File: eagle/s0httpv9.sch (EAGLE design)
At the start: 32 parts, among them X1 MKDSN1,5/6-5,08, X2 MKDSN1,5/6-5,08

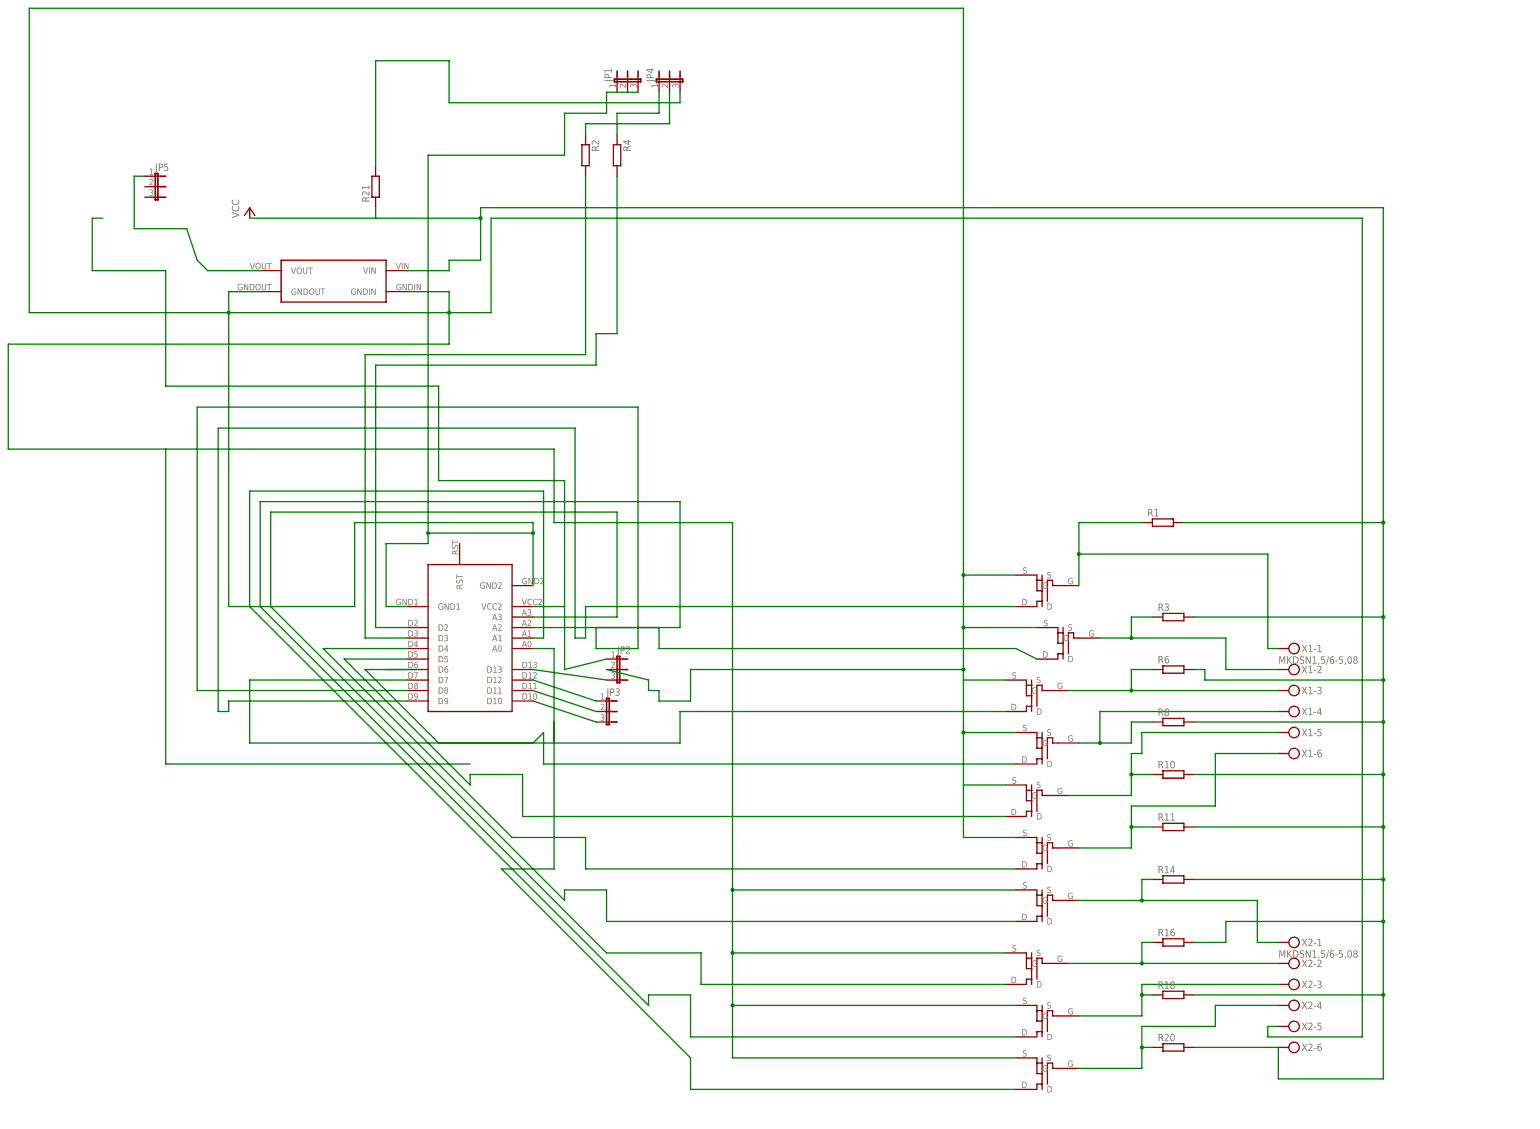
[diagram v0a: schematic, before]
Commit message: schematic cleanup and tagging as v9
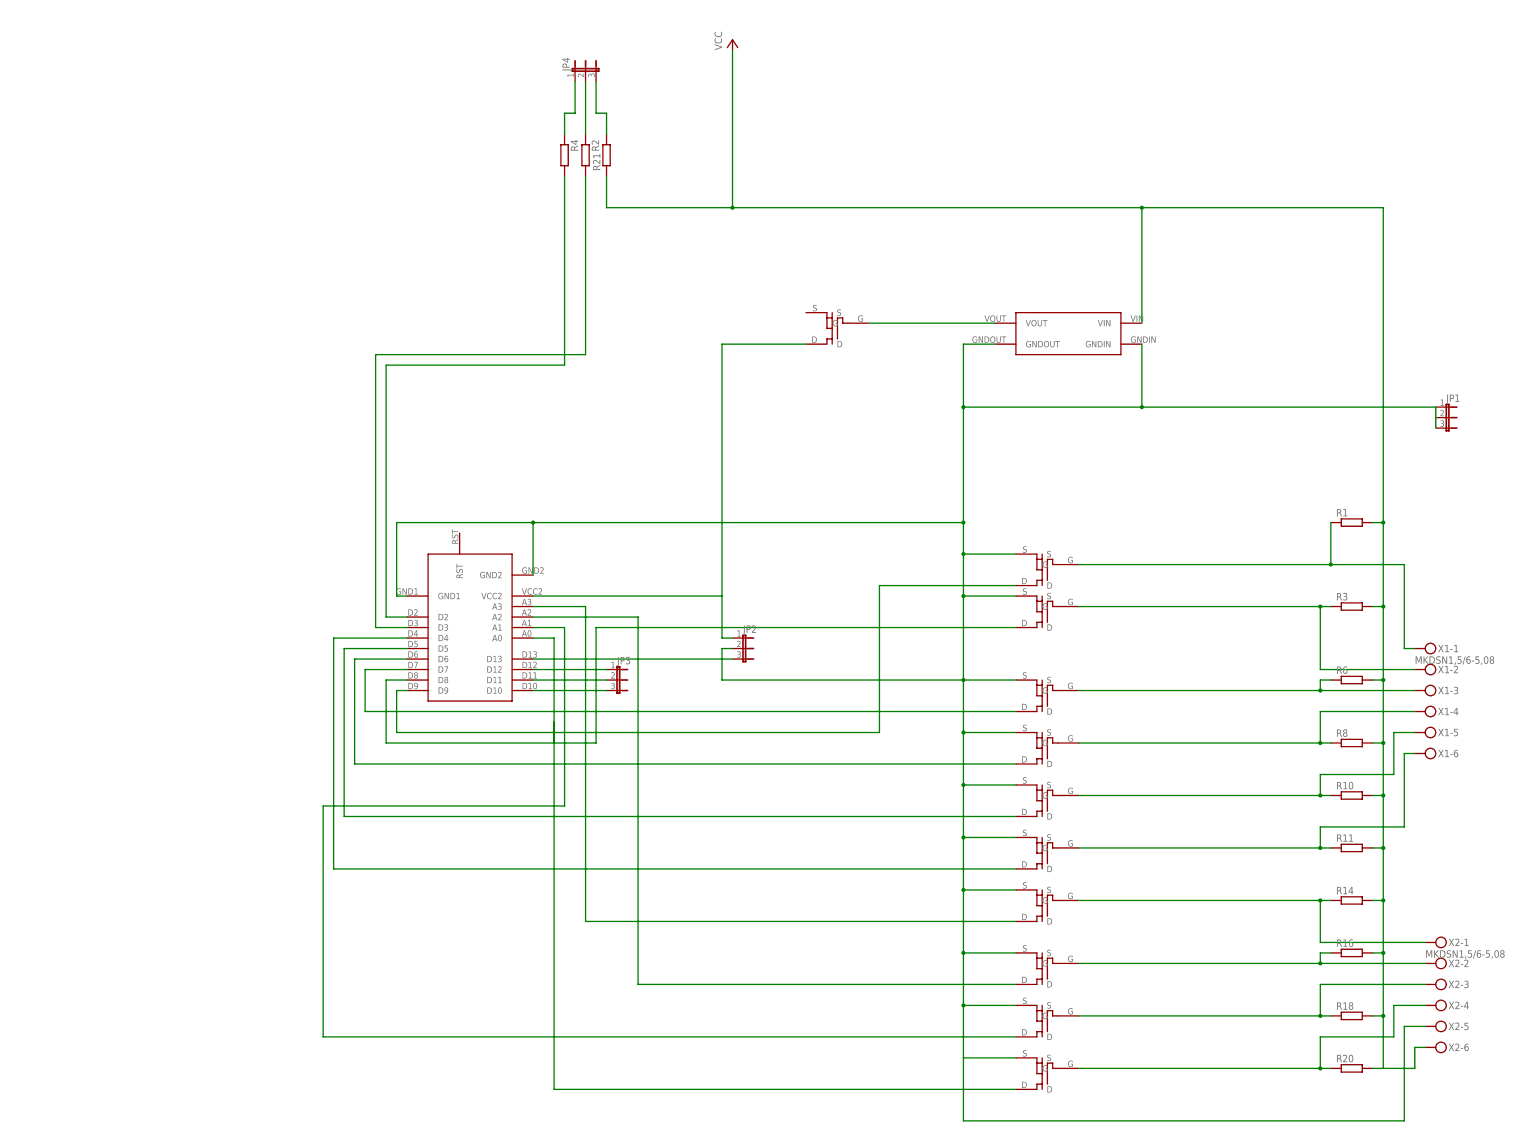
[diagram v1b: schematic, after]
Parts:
- removed JP5: (no value), jumper:JP2E
- added U$13: MOSFET-TO236, snulllib:MOSFET-TO236
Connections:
- net N$12: now also U$13.D
- net N$19: now also U$13.G; no longer JP5.1
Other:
- moved on the sheet: JP1, JP2, JP3, JP4, R1, R10, R11, R14, R16, R18, R20, R21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
